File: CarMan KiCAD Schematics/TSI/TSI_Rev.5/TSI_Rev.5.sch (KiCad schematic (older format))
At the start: 33 parts, among them J1 TSV, J10 J10 GLV PWR, J11 J11 DASH/EPAL, J12 J12 BP SL, J13 J13 RSP SL, J14 Conn_02x05_Odd_Even, J15 J15 ROLL TSAL, J16 J16 THROTTLE PLAUS., J17 J17 BRAKES, J18 J18 RTDS & BRK LIGHT, J19 J19 COOL SENSORS, J2 MC, J20 J20 LSP, J21 J21 I2C, J3 PC Relay, J4 DC Relay, J5 Current_Sensor, J6 J6 IMD, J7 J7 BP CAN & PWR, J8 J8 COCKPIT, J9 J9 COOL PWR, U43 NCD9830DBR2G

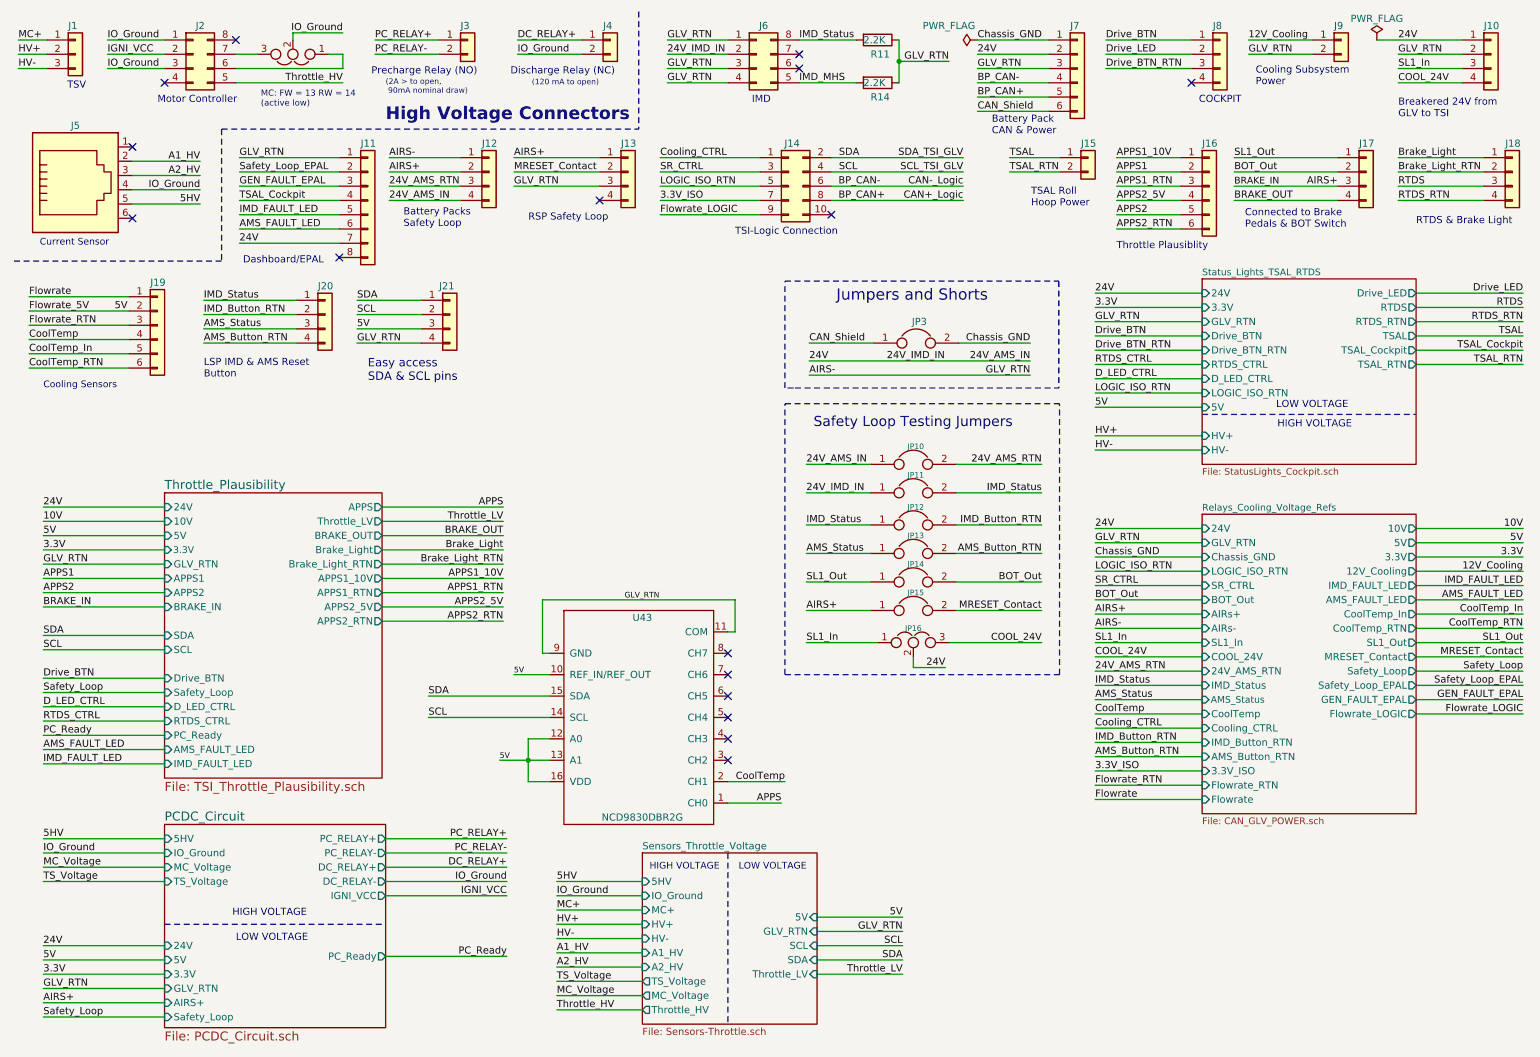
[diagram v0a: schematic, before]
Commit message: Updated TSI Schematic
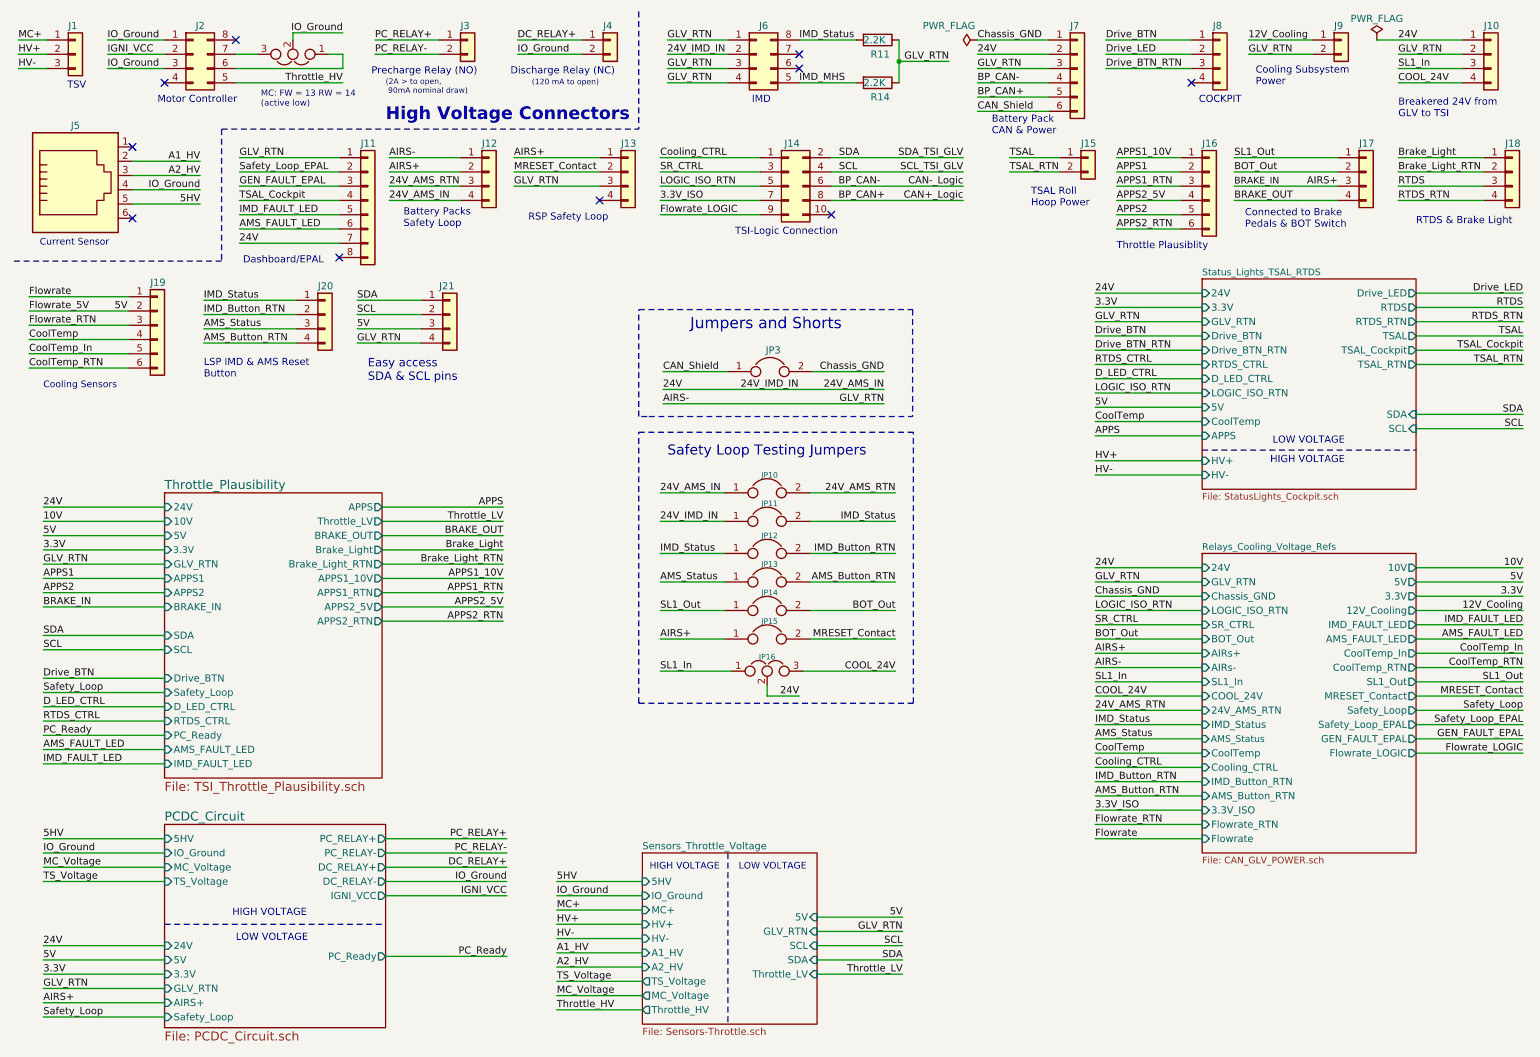
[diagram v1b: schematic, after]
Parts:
- removed U43: NCD9830DBR2G, TSI_Rev_2021_Footprint_Lib:SOP65P640X120-16N, symbol TSI_Rev.5-rescue:NCD9830DBR2G-CarMan_KiCAD_Library-TSI_Rev.5-rescue
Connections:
- no-connect marks 16 -> 10
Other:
- moved on the sheet: JP10, JP11, JP12, JP13, JP14, JP15, JP16, JP3
